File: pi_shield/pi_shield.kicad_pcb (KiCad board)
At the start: 2 copper layers, 56 x 69.3 mm, 31 parts, among them J1 PUMP_NUTRI, J10 1_WIRE, J11 TDS, J12 pH, J2 PUMP_WATER, J3 CLOSURE_WATER, J4 CLOSURE_NUTRI, J5 LEVEL_WATER, J6 LEVEL_NUTRI, J7 Raspberry_Pi_2_3, J8 POWER, J9 12V OUT, SW1 NUTRI_ENA, SW2 WATER_ENA, U1 ATtiny85-20P

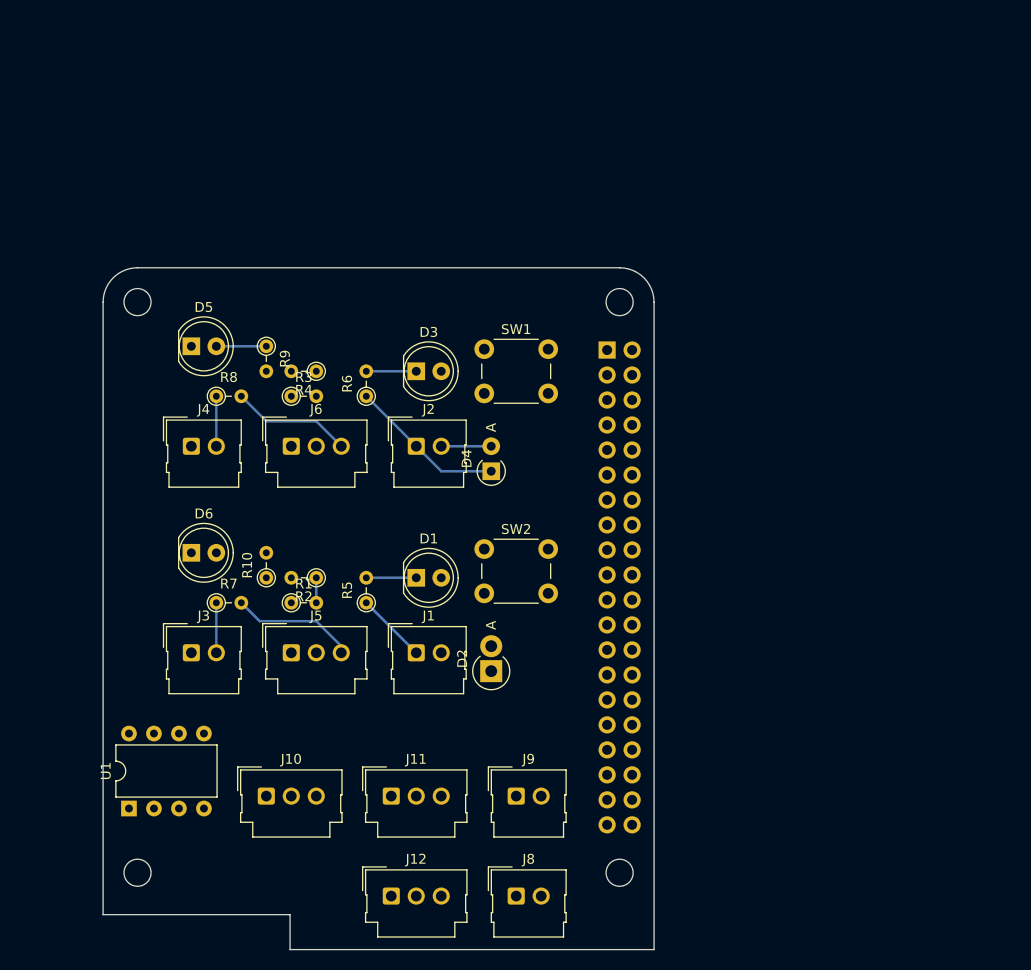
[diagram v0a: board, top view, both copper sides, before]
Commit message: Finish PCBs
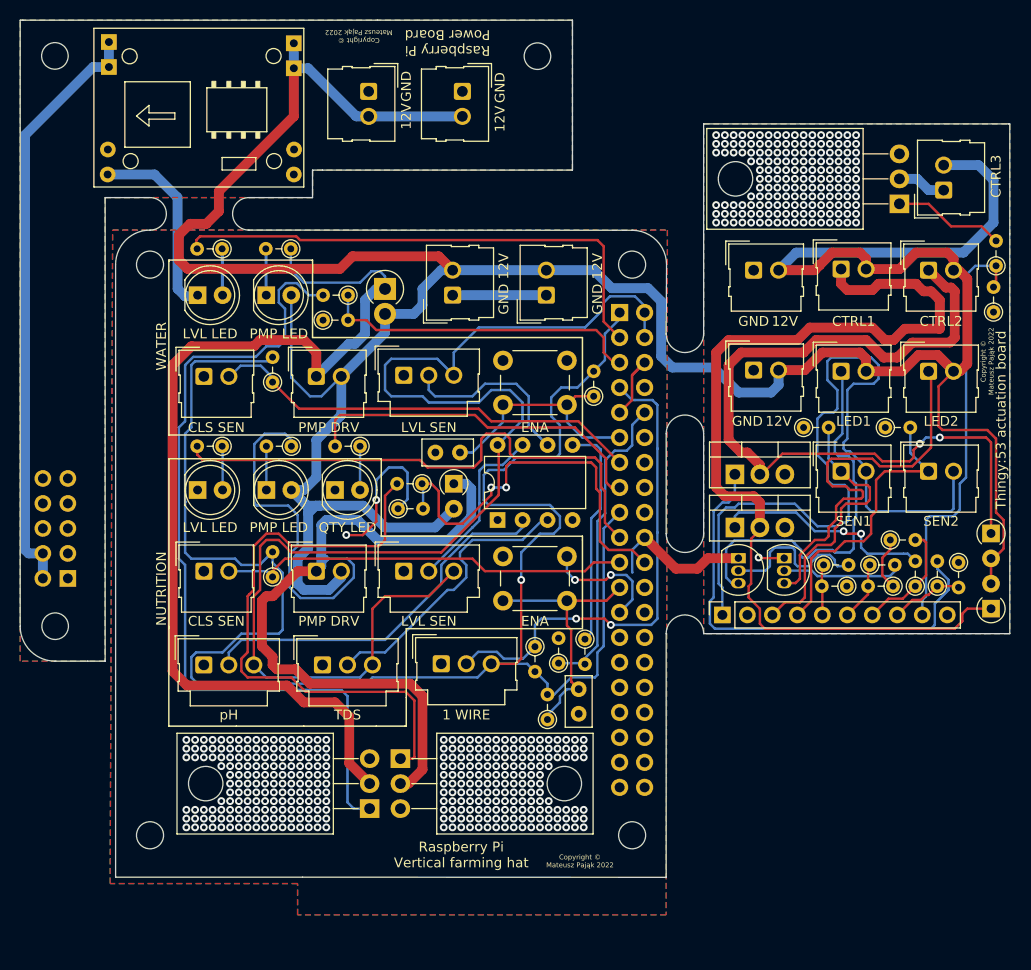
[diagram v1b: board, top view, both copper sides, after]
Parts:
- added C1: C, Capacitor_THT:C_Disc_D5.0mm_W2.5mm_P2.50mm, F.Cu at (161.3, 105.9)
- added C2: C, Capacitor_THT:C_Disc_D5.0mm_W2.5mm_P2.50mm, F.Cu at (146.7, 79.4)
- added D7: LED_NUTRI_QUALITY, LED_THT:LED_D5.0mm_Clear, F.Cu at (136.5, 83.2)
- added D8: DIODE, Diode_THT:D_A-405_P2.54mm_Vertical_AnodeUp, F.Cu at (203.2, 87.6)
- added D9: DIODE, Diode_THT:D_A-405_P2.54mm_Vertical_AnodeUp, F.Cu at (203.2, 95.2)
- added J13: DEBUG CON, Connector_PinSocket_2.54mm:PinSocket_1x10_P2.54mm_Vertical, F.Cu at (175.9, 95.9)
- added J14: LIGHT_SENSOR_2, Connector_Molex:Molex_SL_171971-0002_1x02_P2.54mm_Vertical, F.Cu at (196.8, 81.3)
- added J15: LIGHT_SENSOR_1, Connector_Molex:Molex_SL_171971-0002_1x02_P2.54mm_Vertical, F.Cu at (188.0, 81.3)
- added J16: POWER, Connector_Molex:Molex_SL_171971-0002_1x02_P2.54mm_Vertical, F.Cu at (179.1, 60.8)
- added J17: RELAY_2, Connector_Molex:Molex_SL_171971-0002_1x02_P2.54mm_Vertical, F.Cu at (196.8, 60.8)
- added J18: RELAY_1, Connector_Molex:Molex_SL_171971-0002_1x02_P2.54mm_Vertical, F.Cu at (188.0, 60.7)
- added J19: LED_2, Connector_Molex:Molex_SL_171971-0002_1x02_P2.54mm_Vertical, F.Cu at (196.8, 71.1)
- added J20: LED_1, Connector_Molex:Molex_SL_171971-0002_1x02_P2.54mm_Vertical, F.Cu at (188.0, 71.1)
- added J21: POWER, Connector_Molex:Molex_SL_171971-0002_1x02_P2.54mm_Vertical, F.Cu at (179.1, 71.0)
- added J22: RPI_CON, Connector_PinSocket_2.54mm:PinSocket_2x05_P2.54mm_Vertical, B.Cu at (109.4, 92.2)
- added J23: POWER, Connector_Molex:Molex_SL_171971-0002_1x02_P2.54mm_Vertical, F.Cu at (139.9, 42.7)
- added J24: POWER, Connector_Molex:Molex_SL_171971-0002_1x02_P2.54mm_Vertical, F.Cu at (149.5, 42.7)
- added J25: HEATER_1, Connector_Molex:Molex_SL_171971-0002_1x02_P2.54mm_Vertical, F.Cu at (198.4, 52.7)
- added Q1: IRFZ44N, Package_TO_SOT_THT:TO-220-3_Horizontal_TabDown, F.Cu at (143.2, 110.5)
- added Q2: IRFZ44N, Package_TO_SOT_THT:TO-220-3_Horizontal_TabDown, F.Cu at (140.0, 115.6)
- added Q3: IRFZ44N, Package_TO_SOT_THT:TO-220-3_Vertical, F.Cu at (177.2, 81.6)
- added Q4: IRFZ44N, Package_TO_SOT_THT:TO-220-3_Vertical, F.Cu at (177.2, 87.0)
- added Q5: 2N7000, Package_TO_SOT_THT:TO-92L_Inline, F.Cu at (182.2, 90.1)
- added Q6: 2N7000, Package_TO_SOT_THT:TO-92L_Inline, F.Cu at (177.5, 90.1)
- added Q7: IRFZ44N, Package_TO_SOT_THT:TO-220-3_Horizontal_TabDown, F.Cu at (193.9, 54.1)
- added R11: 10k, Resistor_THT:R_Axial_DIN0204_L3.6mm_D1.6mm_P2.54mm_Vertical, F.Cu at (162.8, 73.7)
- added R12: 10k, Resistor_THT:R_Axial_DIN0204_L3.6mm_D1.6mm_P2.54mm_Vertical, F.Cu at (158.1, 106.5)
- added R13: 4.7k, Resistor_THT:R_Axial_DIN0204_L3.6mm_D1.6mm_P2.54mm_Vertical, F.Cu at (156.8, 99.1)
- added R14: 220R, Resistor_THT:R_Axial_DIN0204_L3.6mm_D1.6mm_P2.54mm_Vertical, F.Cu at (139.1, 78.7)
- added R15: 2k, Resistor_THT:R_Axial_DIN0204_L3.6mm_D1.6mm_P2.54mm_Vertical, F.Cu at (159.2, 100.8)
- added R16: 1k, Resistor_THT:R_Axial_DIN0204_L3.6mm_D1.6mm_P2.54mm_Vertical, F.Cu at (161.9, 98.3)
- added R17: 10k, Resistor_THT:R_Axial_DIN0204_L3.6mm_D1.6mm_P2.54mm_Vertical, F.Cu at (192.5, 76.8)
- added R18: 10k, Resistor_THT:R_Axial_DIN0204_L3.6mm_D1.6mm_P2.54mm_Vertical, F.Cu at (184.2, 76.8)
- added R19: 10k, Resistor_THT:R_Axial_DIN0204_L3.6mm_D1.6mm_P2.54mm_Vertical, F.Cu at (199.9, 90.6)
- added R20: 10k, Resistor_THT:R_Axial_DIN0204_L3.6mm_D1.6mm_P2.54mm_Vertical, F.Cu at (193.0, 88.3)
- added R21: R, Resistor_THT:R_Axial_DIN0204_L3.6mm_D1.6mm_P2.54mm_Vertical, F.Cu at (197.7, 93.0)
- added R22: R, Resistor_THT:R_Axial_DIN0204_L3.6mm_D1.6mm_P2.54mm_Vertical, F.Cu at (195.5, 93.0)
- added R23: 10k, Resistor_THT:R_Axial_DIN0204_L3.6mm_D1.6mm_P2.54mm_Vertical, F.Cu at (193.2, 93.0)
- added R24: 10k, Resistor_THT:R_Axial_DIN0204_L3.6mm_D1.6mm_P2.54mm_Vertical, F.Cu at (188.5, 93.0)
- added R25: R, Resistor_THT:R_Axial_DIN0204_L3.6mm_D1.6mm_P2.54mm_Vertical, F.Cu at (190.9, 90.8)
- added R26: R, Resistor_THT:R_Axial_DIN0204_L3.6mm_D1.6mm_P2.54mm_Vertical, F.Cu at (186.2, 90.8)
- added R27: 10k, Resistor_THT:R_Axial_DIN0204_L3.6mm_D1.6mm_P2.54mm_Vertical, F.Cu at (203.5, 65.1)
- added R28: R, Resistor_THT:R_Axial_DIN0204_L3.6mm_D1.6mm_P2.54mm_Vertical, F.Cu at (203.7, 60.4)
- added REF**: MountingHole_2.7mm, MountingHole:MountingHole_2.7mm, F.Cu at (108.1, 39.1)
- added REF**: MountingHole_2.7mm, MountingHole:MountingHole_2.7mm, F.Cu at (157.1, 39.1)
- added REF**: MountingHole_2.7mm, MountingHole:MountingHole_2.7mm, F.Cu at (108.1, 97.0)
- added U2: STEP_DOWN, Custom:SRT_MPT1584EN_Module, F.Cu at (122.2, 44.9)
- J1: value PUMP_NUTRI -> PUMP_WATER
- J2: value PUMP_WATER -> PUMP_NUTRI
- J9: value 12V OUT -> POWER
- R1, R3, R7, R8: value R -> 10k
- R10, R5, R6, R9: value R -> 220R
- moved J8 61.2 mm to (158.0, 63.4), turned to 90 degrees
- moved J9 51.3 mm to (148.5, 63.4), turned to 90 degrees
- moved U1 47.6 mm to (153.0, 86.2)
- moved D2 40.3 mm to (141.6, 62.8), turned to -90 degrees
- moved R5 36.8 mm to (132.0, 58.7), turned to 180 degrees
- moved R10 33.7 mm to (125.0, 58.7), turned to 180 degrees
- moved D1 32.5 mm to (129.5, 63.4)
- moved J5 30.4 mm to (143.5, 71.5)
- moved J12 30.3 mm to (123.2, 101.0)
- moved J1 29.9 mm to (134.6, 71.6)
- moved R1 28.9 mm to (135.3, 65.9)
- moved R2 28.9 mm to (137.8, 63.4)
- moved J3 28.1 mm to (123.2, 71.6)
- moved D6 26.2 mm to (122.6, 63.4)
- moved R7 23.1 mm to (130.2, 72.2), turned to 90 degrees
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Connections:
- net +12V renamed +12L
- J10 pad 1: unconnected-(J10-Pad1) -> GND
- J10 pad 2: unconnected-(J10-Pad2) -> TEMP
- J10 pad 3: unconnected-(J10-Pad3) -> +3.3V
- J11 pad 1: unconnected-(J11-Pad1) -> GND
- J11 pad 2: unconnected-(J11-Pad2) -> Net-(J11-Pad2)
- J11 pad 3: unconnected-(J11-Pad3) -> +5V
- J12 pad 1: unconnected-(J12-Pad1) -> GND
- J12 pad 2: unconnected-(J12-Pad2) -> Net-(J12-Pad2)
- J12 pad 3: unconnected-(J12-Pad3) -> +5V
- J5 pad 3: +3.3V -> +5V
- J6 pad 3: +3.3V -> +5V
- J7 pad 11: WATER_LED -> WATER_BTN
- J7 pad 12: WATER_CLOSURE -> unconnected-(J7-Pad12)
- J7 pad 13: unconnected-(J7-Pad13) -> WATER_CLOSURE
- J7 pad 15: unconnected-(J7-Pad15) -> NUTRI_QUAL_LED
- J7 pad 19: unconnected-(J7-Pad19) -> NUTRI_LED
- J7 pad 2: unconnected-(J7-Pad2) -> +5V
- J7 pad 21: unconnected-(J7-Pad21) -> NUTRI_CLOSURE
- J7 pad 22: unconnected-(J7-Pad22) -> NUTRI_PUMP
- J7 pad 23: unconnected-(J7-Pad23) -> NUTRI_BTN
- J7 pad 29: NUTRI_LED -> unconnected-(J7-Pad29)
- J7 pad 3: unconnected-(J7-Pad3) -> WATER_LED
- J7 pad 31: NUTRI_CLOSURE -> unconnected-(J7-Pad31)
- J7 pad 4: unconnected-(J7-Pad4) -> +5V
- J7 pad 5: unconnected-(J7-Pad5) -> WATER_PUMP
- J7 pad 7: unconnected-(J7-Pad7) -> TEMP
- R1 pad 2: NUTRI_PUMP -> WATER_PUMP
- R2 pad 1: NUTRI_PUMP -> WATER_PUMP
- R3 pad 2: WATER_PUMP -> NUTRI_PUMP
- R4 pad 1: WATER_PUMP -> NUTRI_PUMP
- SW1 pad 1: unconnected-(SW1-Pad1) -> GND
- SW1 pad 2: unconnected-(SW1-Pad2) -> NUTRI_BTN
- SW2 pad 1: unconnected-(SW2-Pad1) -> GND
- SW2 pad 2: unconnected-(SW2-Pad2) -> WATER_BTN
- U1 pad 2: PIRX -> Net-(J12-Pad2)
- U1 pad 3: unconnected-(U1-Pad3) -> Net-(J11-Pad2)
- U1 pad 5: unconnected-(U1-Pad5) -> Net-(R16-Pad1)
- U1 pad 8: +3.3V -> +5V
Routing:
- net +12L: track 5.08 -> 321.6 mm
- net +3.3V: track 24.9 -> 179.8 mm, vias 0 -> 1
- net +5V: track 0.00 -> 133.1 mm
- net Net-(D9-Pad1): track 0.00 -> 97.5 mm
- net Net-(D2-Pad1): track 7.18 -> 104.7 mm
- net Net-(D4-Pad1): track 15.9 -> 107.0 mm
- net GND: track 0.00 -> 89.3 mm, vias 0 -> 5
- net Net-(Q2-Pad1): track 0.00 -> 85.1 mm
- net Net-(D8-Pad1): track 0.00 -> 82.2 mm, vias 0 -> 2
- net +VDC: track 0.00 -> 82.1 mm
- net +5F: track 0.00 -> 60.6 mm
- net Net-(Q1-Pad1): track 0.00 -> 60.2 mm
- net NUTRI_LED: track 0.00 -> 55.6 mm
- net WATER_LED: track 0.00 -> 52.8 mm
- net TEMP: track 0.00 -> 50.0 mm, vias 0 -> 2
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- added copper zone on B.Cu, net GND
- added copper zone on F.Cu, net GND
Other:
- board size 56 x 69.3 mm -> 100.6 x 87.1 mm
- board text added: "1 WIRE"
- board text added: "12V"
- board text added: "3.3V"
- board text added: "5V"
- board text added: "CLS SEN"
- board text added: "CTRL1"
- board text added: "CTRL2"
- board text added: "CTRL3"
- board text added: "Copyright © Mateusz Pająk 2022"
- board text added: "ENA"
- board text added: "GND"
- board text added: "GND 12V"
- board text added: "LED1"
- board text added: "LED2"
- board text added: "LVL LED"
- board text added: "LVL SEN"
- board text added: "NUTRITION"
- board text added: "PMP DRV"
- board text added: "PMP LED"
- board text added: "QTY LED"
- board text added: "Raspberry Pi Power Board"
- board text added: "Raspberry Pi Vertical farming hat"
- board text added: "SEN1"
- board text added: "SEN2"
- board text added: "SIG"
- board text added: "TDS"
- board text added: "Thingy:53 actuation board"
- board text added: "WATER"
- board text added: "https://github.com/Tai-Min/Aeroponic-Garden-System"
- board text added: "pH"
